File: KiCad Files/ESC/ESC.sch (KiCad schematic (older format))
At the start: 97 parts, among them J1 Conn_01x03, J10 Conn_01x03, J11 Conn_01x04, J2 Conn_01x06_Female, J3 Conn_01x01, J4 Conn_01x01, J5 Conn_01x01, J6 Conn_01x03, J7 Conn_01x02, J8 Conn_01x04, J9 Conn_01x03, Q1 IRF3205, Q2 IRF3205, Q3 IRF3205, Q4 IRF3205, Q5 IRF3205, Q6 IRF3205, U1 LM339, U2 L7809, U3 MCP601-xP, U4 IR2110, U5 IR2110, U6 IR2110

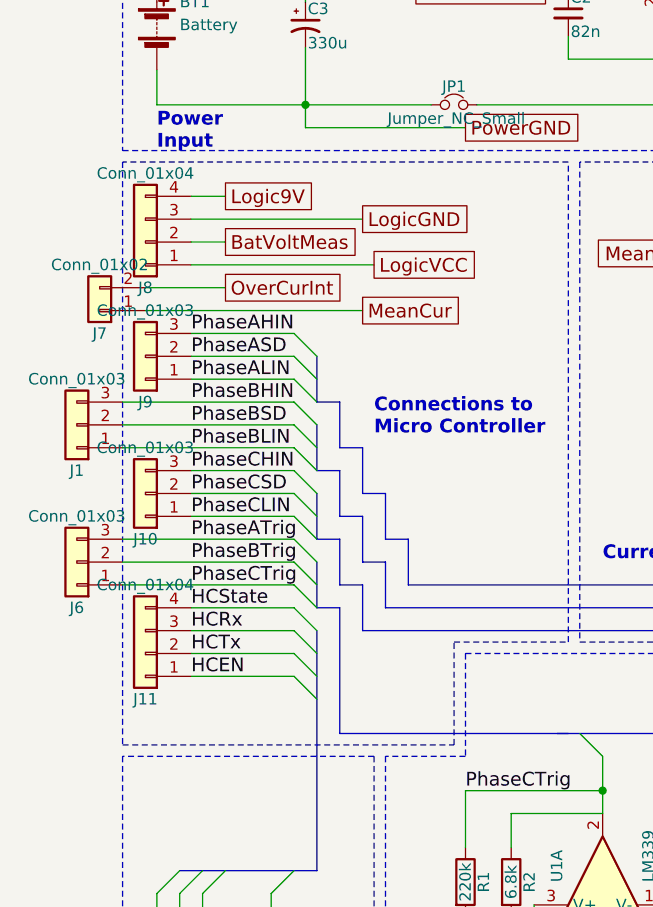
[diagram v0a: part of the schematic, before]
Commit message: Finished PCB v1 and Started v2
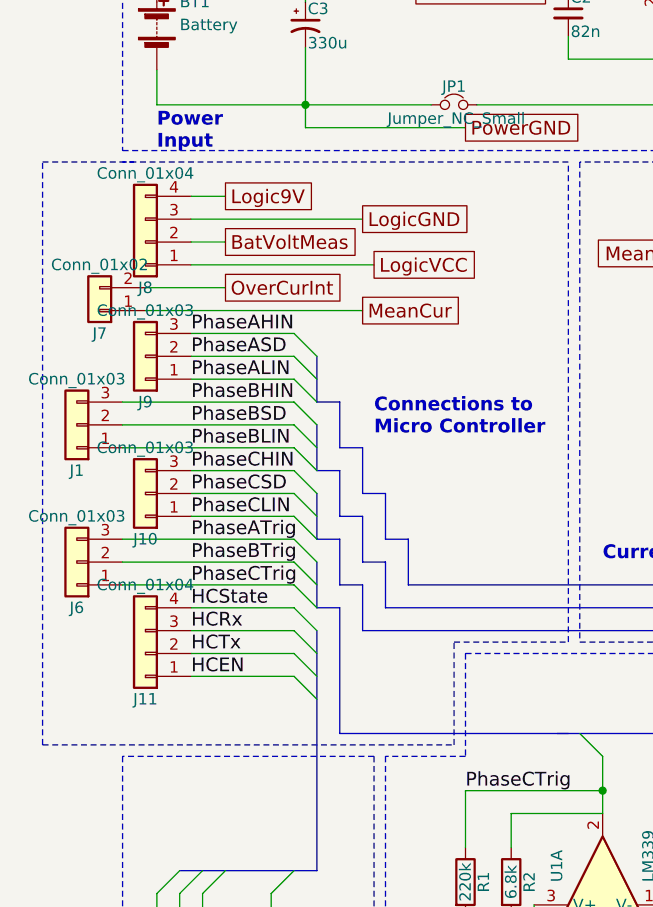
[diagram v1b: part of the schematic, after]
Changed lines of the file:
@@
 	10650 2350 6100 2350
 Wire Notes Line
-	850  1750 850  4300
-Wire Notes Line
-	850  4300 2300 4300
+	500  4300 2300 4300
 Wire Notes Line
 	850  550  4150 550
@@
 	-1   0    0    1
 $EndComp
+Wire Notes Line
+	500  4300 500  1750
+Wire Notes Line
+	500  1750 900  1750
 $EndSCHEMATC
